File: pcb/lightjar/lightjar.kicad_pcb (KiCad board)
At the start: 2 copper layers, 21 parts, among them J1 Power/Comms, J2 Button, J3 Photoresistor, J4 Potentiometer, Q1 MMBTA42, U1 AMS1117-5.0, U2 Pico

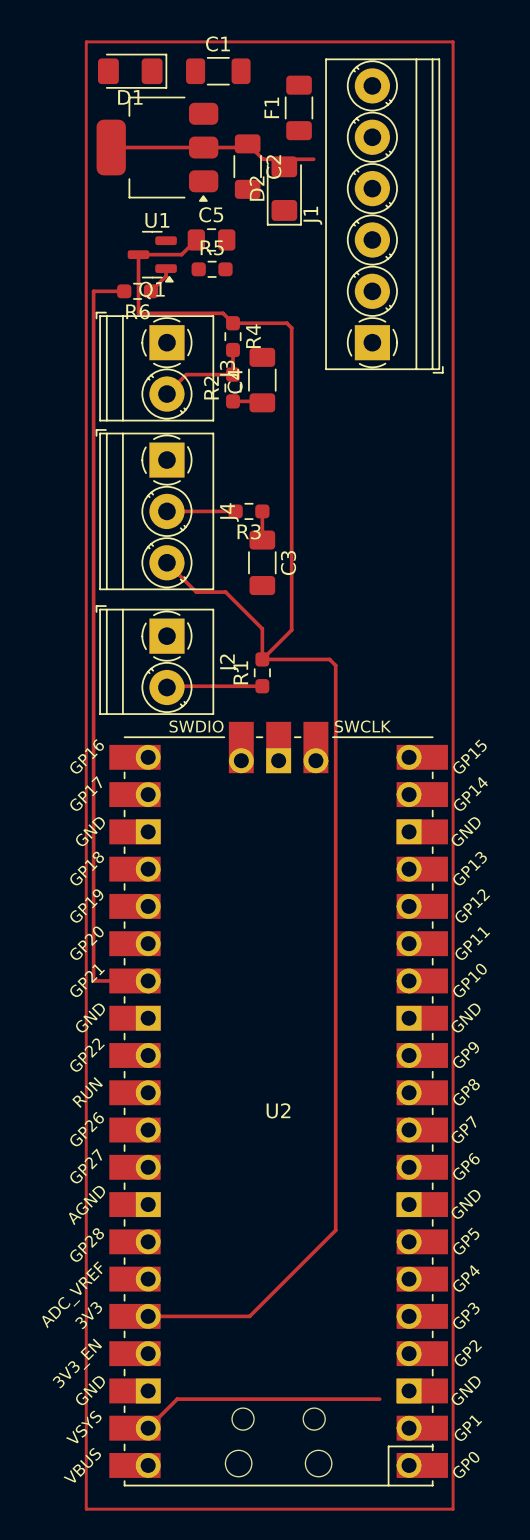
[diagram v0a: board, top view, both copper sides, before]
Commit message: Layout and schematic updates
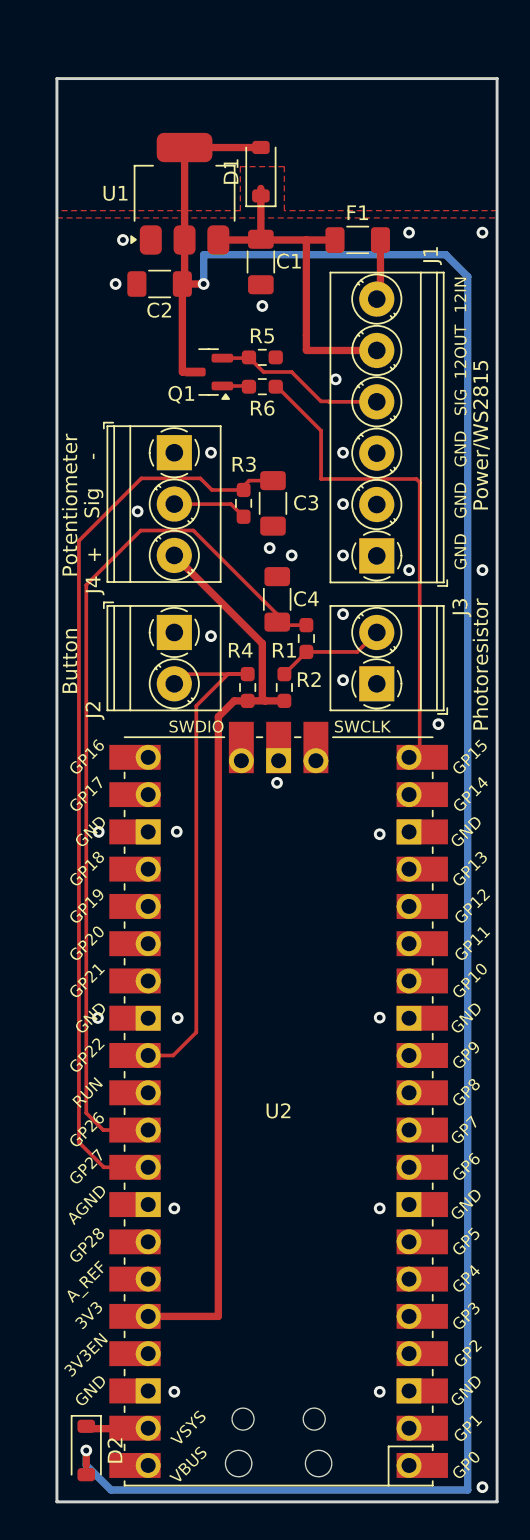
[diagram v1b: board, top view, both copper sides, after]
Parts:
- removed C5: 0.1 uF, Capacitor_SMD:C_0805_2012Metric_Pad1.18x1.45mm_HandSolder
- D1, D2: footprint Diode_SMD:D_1206_3216Metric_Pad1.42x1.75mm_HandSolder -> Diode_SMD:D_SOD-123
- R6: value 125 -> 220
- moved D2 87.1 mm to (150.0, 126.0), turned to -90 degrees
- moved J3 27.3 mm to (169.8, 73.8), turned to 90 degrees
- moved R4 24.2 mm to (163.5, 74.0), turned to 90 degrees
- moved R2 17.8 mm to (165.0, 70.7), turned to -90 degrees
- moved C4 15.0 mm to (163.0, 68.0)
- moved J1 14.5 mm to (169.8, 65.0)
- moved C1 13.3 mm to (161.9, 45.0), turned to -90 degrees
- moved D1 11.2 mm to (161.9, 38.8), turned to 90 degrees
- moved R6 10.7 mm to (162.0, 53.5), turned to 0 degrees
- moved C2 10.0 mm to (155.0, 46.5), turned to 180 degrees
- moved F1 9.85 mm to (168.5, 43.5), turned to 0 degrees
- moved Q1 8.87 mm to (158.3, 52.5)
- moved R5 6.91 mm to (162.0, 51.5)
- moved C3 4.11 mm to (162.7, 61.5)
- moved U1 3.65 mm to (156.7, 40.4), turned to 90 degrees
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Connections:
- C3 pad 1: Brightness -> Brightness Pin
- C4 pad 1: Photoresistor -> Photoresistor Pin
- Q1 pad 2: WS2315 Output -> WS2815 Output
- Q1 pad 3: +3.3V -> +5V
- R2 pad 1: Photoresistor -> Photoresistor Pin
- R3 pad 1: Brightness -> Brightness Pin
- R5 pad 1: WS2315 Output -> WS2815 Output
- U2 pad 20: unconnected-(U2-GPIO15-Pad20) -> WS2815 Pin
- U2 pad 27: WS2815 Pin -> unconnected-(U2-GPIO21-Pad27)
- U2 pad 31: unconnected-(U2-GPIO26_ADC0-Pad31) -> Photoresistor Pin
- U2 pad 32: Photoresistor -> Brightness Pin
- U2 pad 34: Brightness -> unconnected-(U2-GPIO28_ADC2-Pad34)
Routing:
- net +5V: track 14.3 -> 155.0 mm, vias 0 -> 2
- net Brightness Pin: track 0.00 -> 62.2 mm
- net Photoresistor Pin: track 0.00 -> 60.2 mm
- net +3.3V: track 111.9 -> 63.1 mm
- net Button Sig: track 6.54 -> 35.9 mm
- net +12V: track 0.00 -> 23.8 mm
- net WS2815 Pin: track 52.8 -> 33.5 mm
- net Net-(D2-K): track 16.6 -> 4.23 mm
- net WS2815 Output: track 0.00 -> 11.8 mm
- net +12VA: track 0.00 -> 4.13 mm
- net Photoresistor: track 2.04 -> 0.00 mm
- net Brightness: track 1.95 -> 0.00 mm
- net Photoresistor Sig: track 6.72 -> 7.48 mm
- net GND: vias 0 -> 31
- added copper zone on F.Cu, net +5V
- added copper zone on B.Cu, net GND
- added copper zone on F.Cu, net GND
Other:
- board outline added: 30 x 97 mm
- board text added: "+"
- board text added: "-"
- board text added: "12IN"
- board text added: "12OUT"
- board text added: "Button"
- board text added: "GND"
- board text added: "Photoresistor"
- board text added: "Potentiometer"
- board text added: "Power/WS2815"
- board text added: "SIG"
- board text added: "Sig"
